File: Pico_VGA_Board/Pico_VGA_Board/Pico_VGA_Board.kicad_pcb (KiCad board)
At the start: 2 copper layers, 108 x 58.4 mm, 51 parts, among them IC1 NC7WZ17P6X, J1 DE15_Plug_HighDensity, J2 Micro_SD_Card_Det1, J3 AudioJack3, SW1 SW_MEC_5E, U1 Pico

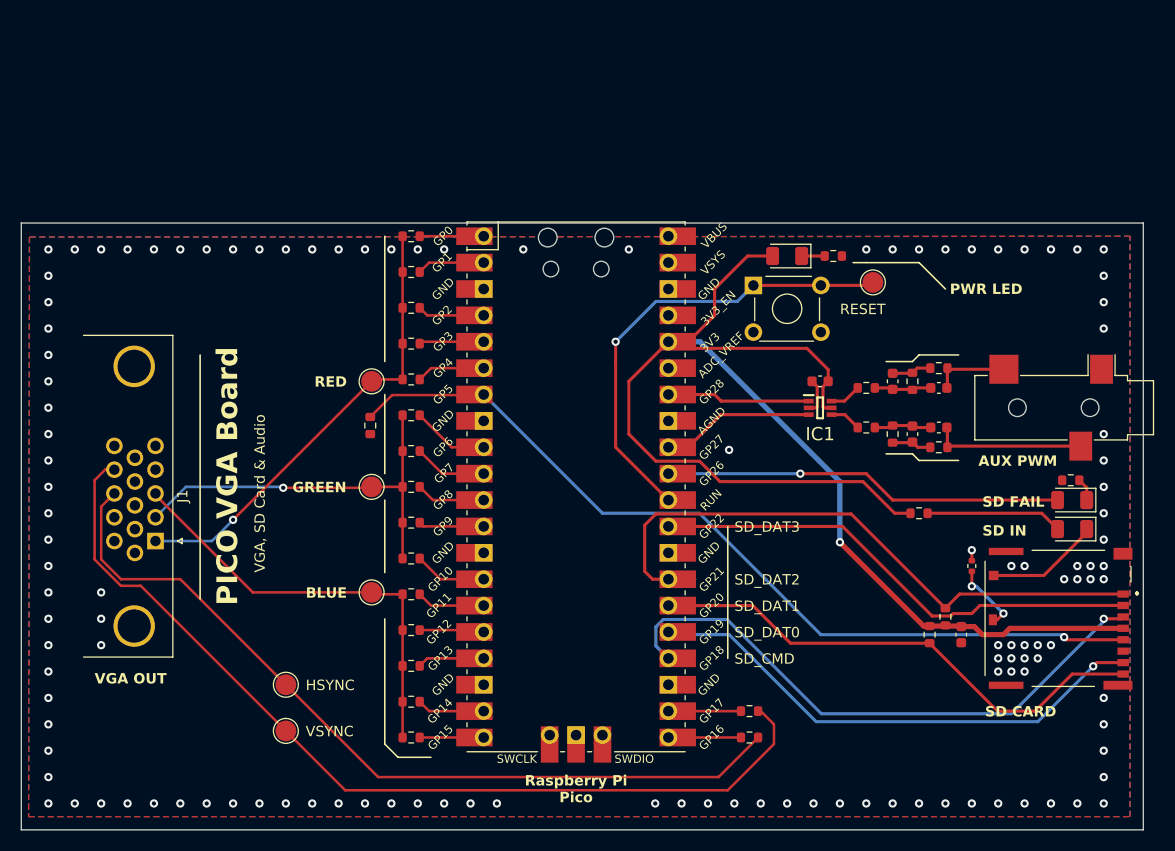
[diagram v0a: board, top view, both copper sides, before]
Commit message: UPD Board
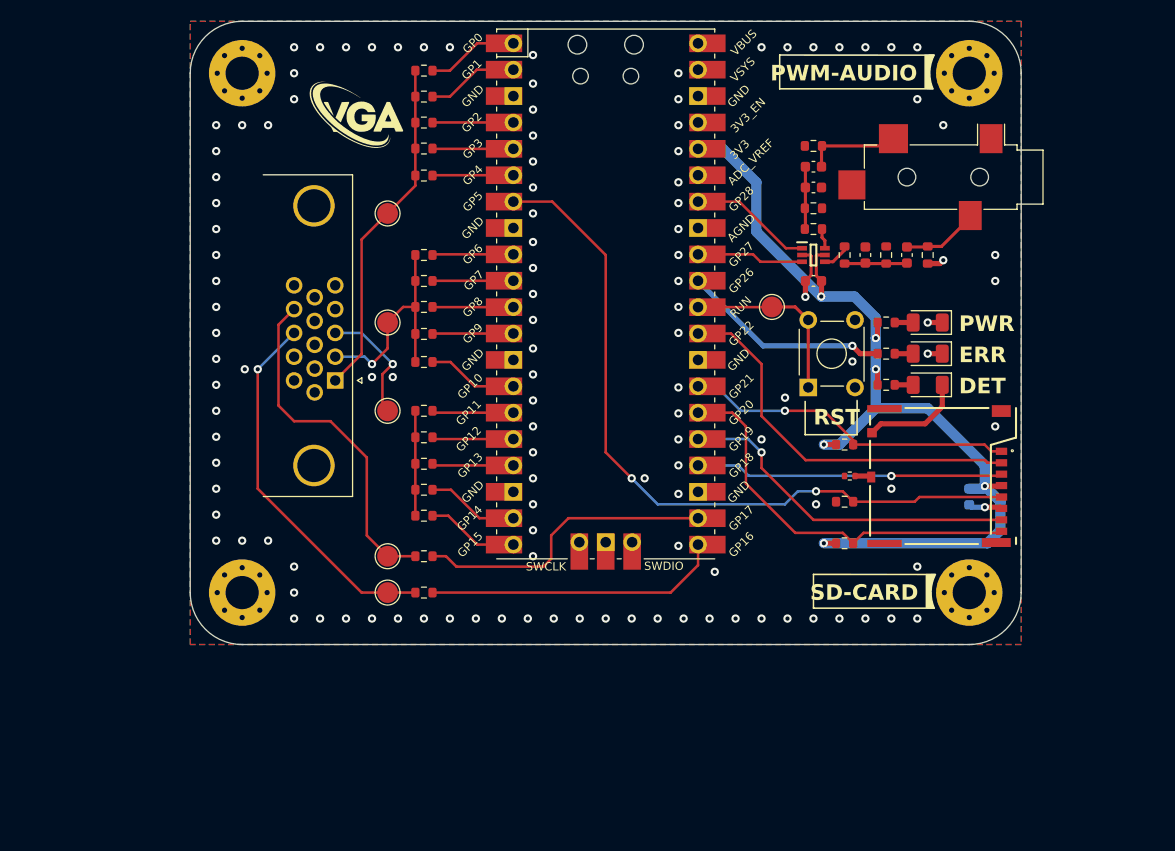
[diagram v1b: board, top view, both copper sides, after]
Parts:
- added G***: LOGO, Symbol:VGA, F.Cu at (131.0, 64.0)
- added H1: MountingHole_Pad, MountingHole:MountingHole_3.2mm_M3_Pad_Via, F.Cu at (120.0, 60.0)
- added H2: MountingHole_Pad, MountingHole:MountingHole_3.2mm_M3_Pad_Via, F.Cu at (190.0, 60.0)
- added H3: MountingHole_Pad, MountingHole:MountingHole_3.2mm_M3_Pad_Via, F.Cu at (120.0, 110.0)
- added H4: MountingHole_Pad, MountingHole:MountingHole_3.2mm_M3_Pad_Via, F.Cu at (190.0, 110.0)
- C1: moved to B.Cu
- IC1: footprint Samacsys:SOP65P210X110-6N -> Package_SO:SOP65P210X110-6N
- J2: footprint Samacsys:5033981892 -> SamacSys_Parts:503398-1892
- J3: footprint Connector_Audio:Jack_3.5mm_CUI_SJ-3523-SMT_Horizontal -> Connector_Audio:Jack_3.5mm_CUI_SJ-3524-SMT_Horizontal
- U1: footprint Pico_W:RPi_Pico_SMD_TH -> Module:RPi_Pico_SMD_TH
- moved R20 46.3 mm to (178.0, 101.2), turned to 180 degrees
- moved R17 34.7 mm to (137.5, 106.5), turned to 180 degrees
- moved R16 34.3 mm to (137.5, 110.0), turned to 180 degrees
- moved J3 24.6 mm to (188.5, 70.0)
- moved R29 24.6 mm to (175.0, 67.0)
- moved C6 24.5 mm to (175.0, 69.0)
- moved J1 23.2 mm to (129.0, 89.6)
- moved R30 21.5 mm to (182.0, 87.0), turned to 0 degrees
- moved R11 21.4 mm to (137.5, 102.6)
- moved J2 20.8 mm to (194.5, 92.2)
- moved R12 20.4 mm to (137.5, 100.1)
- moved C5 20.2 mm to (175.0, 71.0), turned to 0 degrees
- moved D3 19.8 mm to (186.0, 87.0)
- moved R1 19.7 mm to (137.5, 69.8)
- moved D1 19.6 mm to (186.0, 90.0)
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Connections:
- D2 pad 1: Net-(D2-K) -> GND
- D2 pad 2: +3V3 -> Net-(D2-A)
- D3 pad 1: Net-(D3-K) -> GND
- D3 pad 2: /SD_ERR_LED -> Net-(D3-A)
- R23 pad 1: Net-(D2-K) -> Net-(D2-A)
- R23 pad 2: GND -> +3V3
- R30 pad 1: Net-(D3-K) -> /SD_ERR_LED
- R30 pad 2: GND -> Net-(D3-A)
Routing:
- net /VSYNC: track 90.4 -> 33.5 mm
- net /HSYNC: track 80.4 -> 35.8 mm, vias 0 -> 1
- net +3V3: track 135.9 -> 92.7 mm, vias 1 -> 6
- net /SD_DAT2: track 60.4 -> 32.4 mm, vias 0 -> 1
- net /SD_CMD: track 56.6 -> 29.7 mm
- net Net-(U1-RUN): track 44.5 -> 17.6 mm, vias 1 -> 0
- net Net-(U1-GPIO17): track 6.98 -> 29.2 mm
- net Net-(U1-GPIO16): track 6.98 -> 28.6 mm
- net /VGA_B: track 41.9 -> 22.0 mm, vias 0 -> 1
- net /SD_ERR_LED: track 38.5 -> 20.2 mm
- net /SD_DAT0: track 49.7 -> 33.3 mm
- net /VGA_G: track 38.9 -> 22.6 mm
- net /SD_CLK: track 83.2 -> 71.3 mm, vias 1 -> 2
- net Net-(D1-A): track 13.1 -> 1.78 mm
- net /SD_DAT1: track 49.5 -> 38.1 mm
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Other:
- board size 108 x 58.4 mm -> 80 x 60 mm
- board text added: "DET"
- board text added: "ERR"
- board text added: "PWM-AUDIO"
- board text added: "PWR"
- board text added: "RST"
- board text added: "SD-CARD"
- board text removed: "AUX PWM"
- board text removed: "BLUE"
- board text removed: "GREEN"
- board text removed: "HSYNC"
- board text removed: "PICO VGA Board"
- board text removed: "PWR LED"
- board text removed: "RED"
- board text removed: "RESET"
- board text removed: "Raspberry Pi Pico"
- board text removed: "SD CARD"
- board text removed: "SD FAIL"
- board text removed: "SD IN"
- board text removed: "SD_CMD"
- board text removed: "SD_DAT0"
- board text removed: "SD_DAT1"
- board text removed: "SD_DAT2"
- board text removed: "SD_DAT3"
- board text removed: "VGA OUT"
- board text removed: "VGA, SD Card & Audio"
- board text removed: "VSYNC"
